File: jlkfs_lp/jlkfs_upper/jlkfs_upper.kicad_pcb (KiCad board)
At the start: 2 copper layers, 142.5 x 133.4 mm, 38 parts, among them J0 USB_C_Receptacle_PowerOnly_6P, SW0 SWITCH, SW1 SWITCH, SW10 SWITCH, SW11 SWITCH, SW12 SWITCH, SW13 SWITCH, SW14 SWITCH, SW15 SWITCH, SW16 SWITCH, SW17 SWITCH, SW18 SWITCH, SW19 SWITCH, SW2 SWITCH, SW20 SWITCH, SW21 SWITCH, SW22 SWITCH, SW23 SWITCH, SW24 SWITCH, SW25 SWITCH, SW26 SWITCH, SW27 SWITCH, SW28 SWITCH, SW3 SWITCH, SW4 SWITCH, SW5 SWITCH, SW6 SWITCH, SW7 SWITCH, SW8 SWITCH, SW9 SWITCH, U0 RP2040

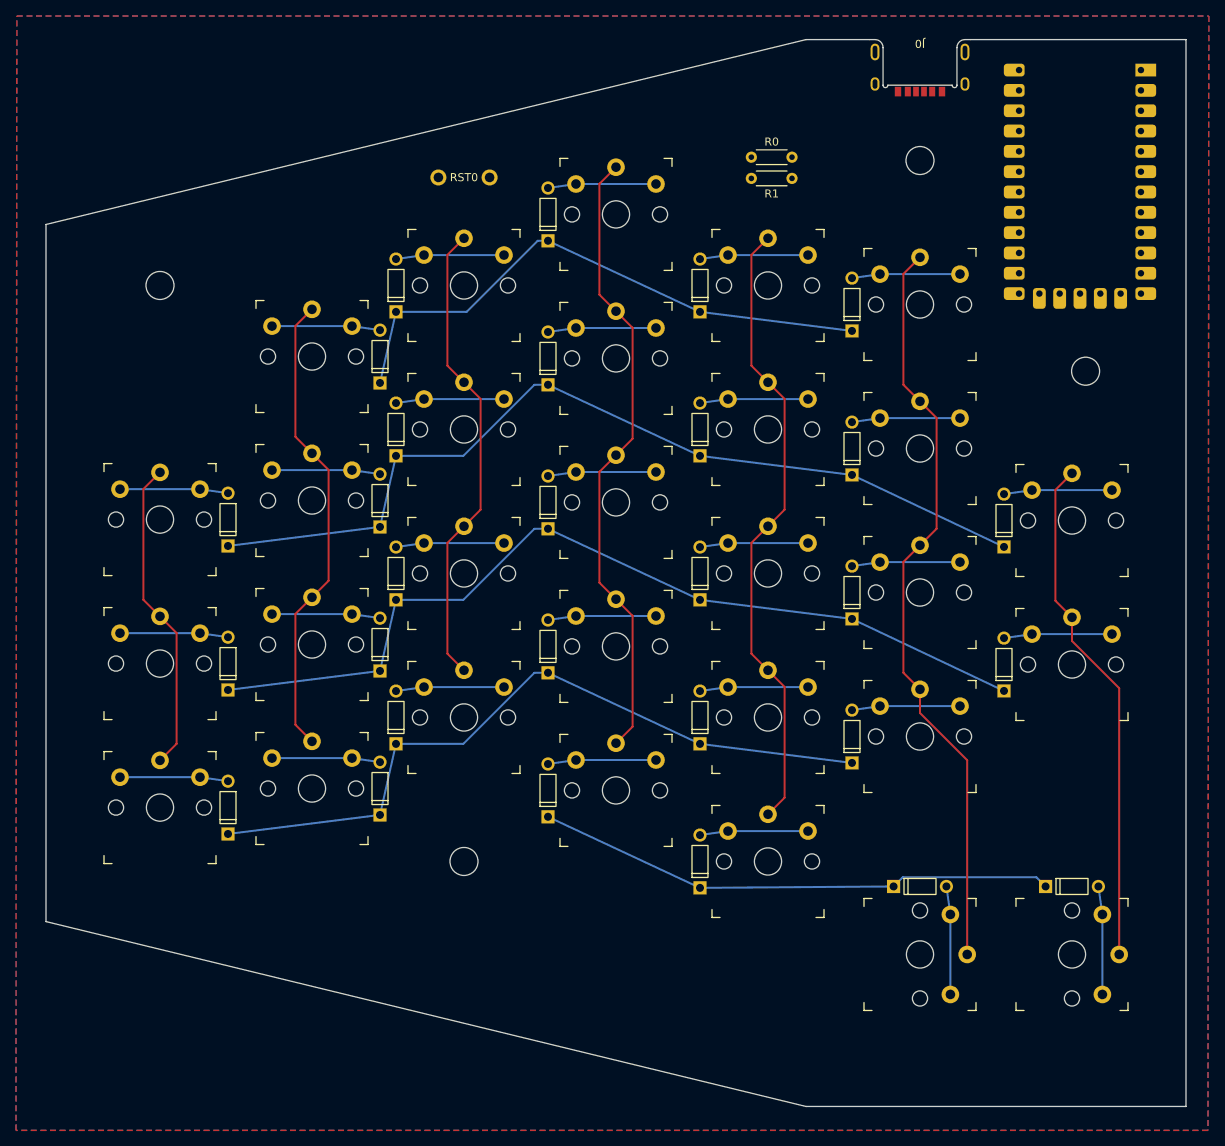
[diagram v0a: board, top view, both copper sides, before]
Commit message: Updated jlkfs_lp.
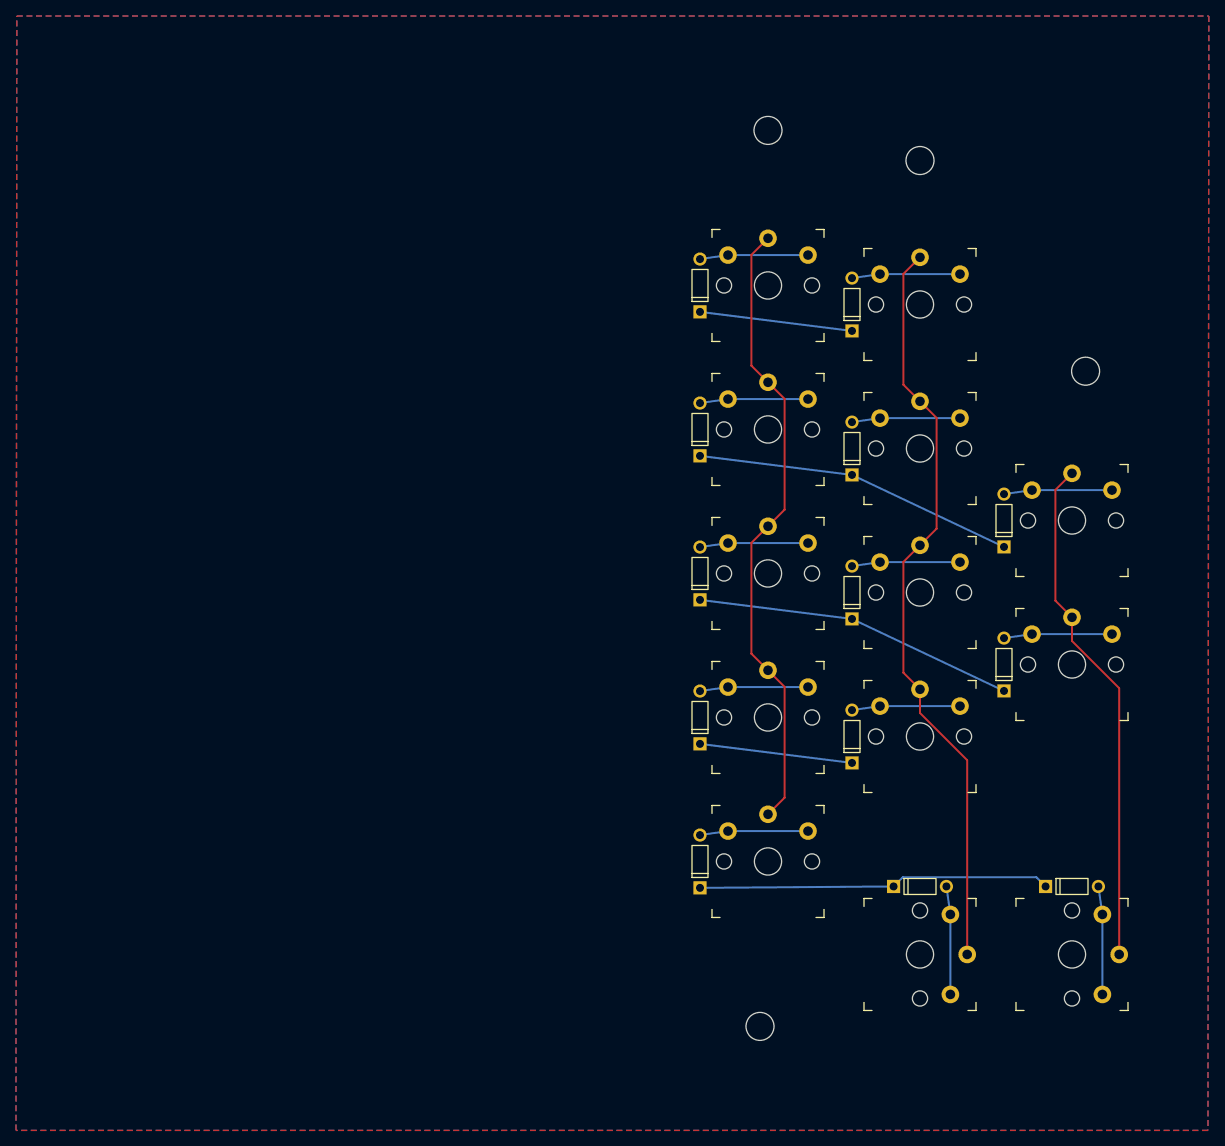
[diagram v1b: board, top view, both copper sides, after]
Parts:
- removed J0: USB_C_Receptacle_PowerOnly_6P, footprints:USB4515
- removed R0, R1: R, Resistor_THT:R_Axial_DIN0204_L3.6mm_D1.6mm_P5.08mm_Horizontal
- removed RST0: SW_Push, footprints:reset_button
- removed SW0, SW1, SW12, SW13, SW14, SW15, SW19, SW2, SW20, SW21, SW22, SW25, SW5, SW6, SW7, SW8: SWITCH, footprints:kailh_choc_dual_with_diode
- removed U0: RP2040, footprints:pro_micro_castellated
- moved H3 78.4 mm to (167.0, 30.0)
- moved H2 42.4 mm to (166.0, 142.0)
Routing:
- net /COL3: track 78.9 -> 0.00 mm
- net /ROW2: track 112.1 -> 40.2 mm
- net /ROW1: track 112.1 -> 40.2 mm
- net /ROW3: track 91.1 -> 19.1 mm
- net /COL5: track 59.2 -> 0.00 mm
- net /COL4: track 59.2 -> 0.00 mm
- net /ROW0: track 71.9 -> 19.1 mm
- net /COL6: track 39.4 -> 0.00 mm
- net /ROW4: track 65.1 -> 44.2 mm
- net Net-(SW8-A): track 13.5 -> 0.00 mm
- net Net-(SW7-A): track 13.5 -> 0.00 mm
- net Net-(SW6-A): track 13.5 -> 0.00 mm
- net Net-(SW5-A): track 13.5 -> 0.00 mm
- net Net-(SW25-A): track 13.5 -> 0.00 mm
- net Net-(SW22-A): track 13.5 -> 0.00 mm
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- added copper zone on B.Cu, net (none)
- added copper zone on F.Cu, net (none)
- removed copper zone on B.Cu, net GND
- removed copper zone on F.Cu, net GND
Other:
- board outline removed
